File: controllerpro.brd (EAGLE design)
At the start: 85.1 x 38.7 mm, 10 parts, among them IC1 MCP1703CB, IC2 741G3157DBVR, IC3 741G3157DBVR, IC4 741G3157DBVR, IC5 741G3157DBVR

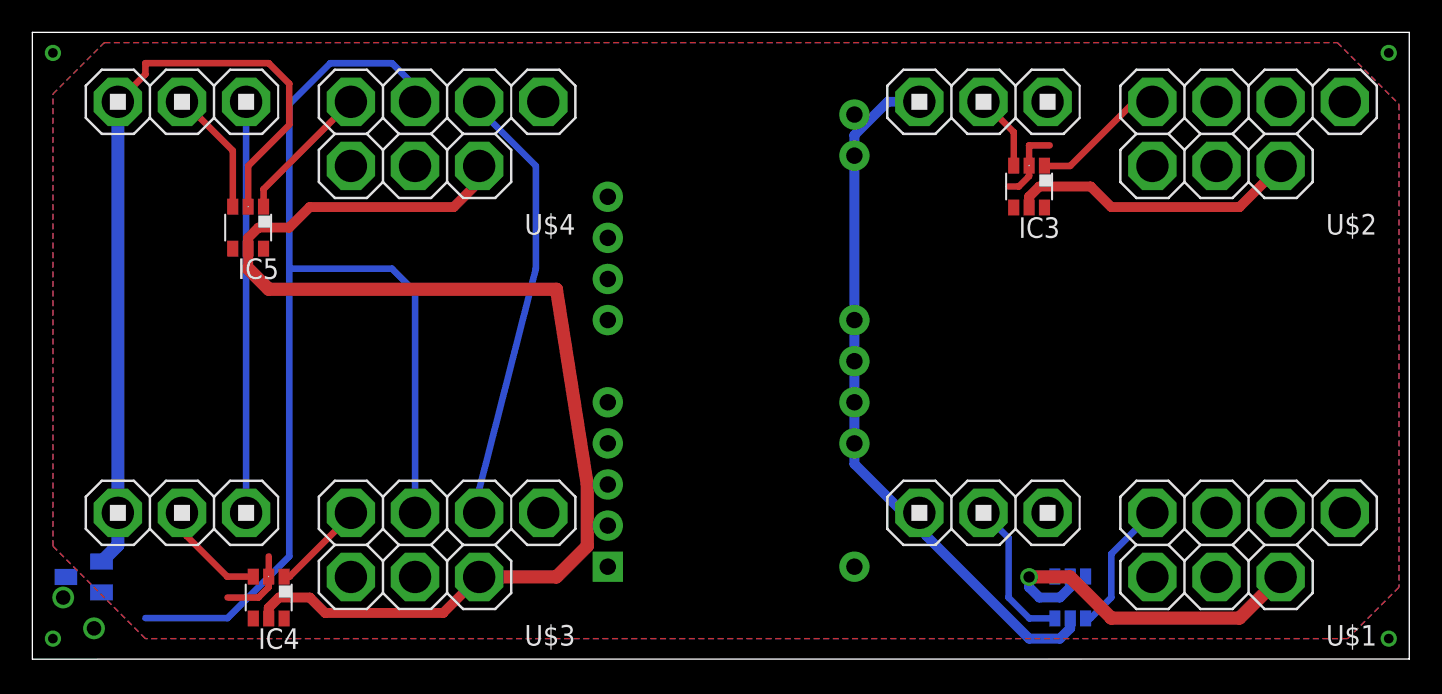
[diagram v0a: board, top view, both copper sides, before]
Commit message: All wired up (intially)!
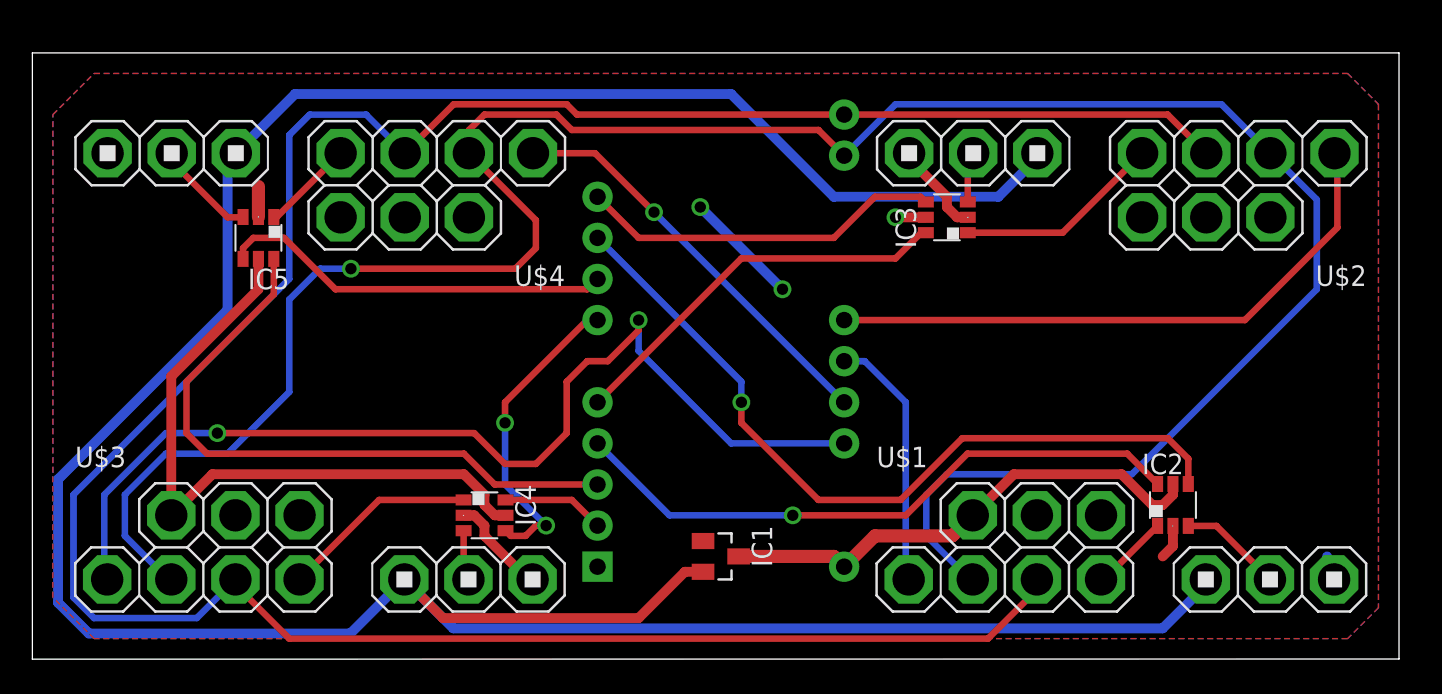
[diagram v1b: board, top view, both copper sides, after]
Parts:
- moved IC1 39.4 mm to (42.5, 6.35), flipped to the top
- moved IC4 14.3 mm to (27.9, 8.89), turned to 270 degrees
- moved IC2 8.54 mm to (70.5, 9.53), flipped to the top
- moved IC3 5.43 mm to (56.5, 27.3), turned to 90 degrees
- moved U$1 4.96 mm to (66.0, 8.89), turned to 0 degrees
- moved U$3 4.96 mm to (16.5, 8.89), turned to 0 degrees
- moved U$2 3.24 mm to (68.6, 27.3)
- moved U$4 3.24 mm to (19.1, 27.3)
- moved IC5 0.90 mm to (14.0, 26.0)
- moved U$5 0.63 mm to (42.5, 19.7)
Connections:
- net DATA0: now also U$5.D2; no longer U$5.D3
- net DATA1: now also U$5.D3; no longer U$5.D2
- net DATA2: now also U$5.D0; no longer U$5.D1
- net DATA3: now also U$5.D1; no longer U$5.D0
- net N64_OR_NES0: now also U$5.B2; no longer U$5.B3
- net N64_OR_NES1: now also U$5.B3; no longer U$5.B2
- net N64_OR_NES2: now also U$5.B0; no longer U$5.B1
- net N64_OR_NES3: now also U$5.B1; no longer U$5.B0
- net S_OR_NES0: now also U$5.F6; no longer U$5.F7
- net S_OR_NES1: now also U$5.F7; no longer U$5.F6
- net S_OR_NES2: now also U$5.F4; no longer U$5.F5
- net S_OR_NES3: now also U$5.F5; no longer U$5.F4
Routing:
- net V33: track 25.4 -> 183.7 mm
- net CLOCK: track 27.3 -> 149.8 mm, vias 0 -> 1
- net LATCH: track 70.8 -> 159.4 mm
- net GND: track 104.0 -> 25.8 mm, vias 0 -> 2
- net S_OR_NES2: track 0.00 -> 63.6 mm, vias 0 -> 2
- net DATA0: track 0.00 -> 48.4 mm, vias 0 -> 1
- net VCC: track 117.3 -> 74.6 mm
- net N64_OR_NES3: track 0.00 -> 39.7 mm
- net N64_OR_NES0: track 0.00 -> 38.8 mm, vias 0 -> 1
- net S_OR_NES1: track 0.00 -> 37.5 mm
- net S_OR_NES3: track 0.00 -> 25.6 mm, vias 0 -> 1
- net N64_OR_NES1: track 0.00 -> 24.6 mm
- net DATA3: track 0.00 -> 24.4 mm
- net DATA1: track 0.00 -> 22.5 mm
- net DATA2: track 0.00 -> 19.4 mm, vias 0 -> 2
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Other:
- board size 85.1 x 38.7 mm -> 84.5 x 37.5 mm
